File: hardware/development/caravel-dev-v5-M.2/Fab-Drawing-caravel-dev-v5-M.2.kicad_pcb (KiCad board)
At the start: 2 copper layers, 76.2 x 73.8 mm, 70 parts, among them J1 USB_B_Micro, J10 Conn_01x28_Pin, J11 Conn_01x28_Pin, J12 Conn_01x04_Pin, J2 Conn_01x02_Pin, J3 Conn_01x02_Pin, J4 Conn_01x03_Pin, J5 Conn_01x02_Pin, J6 Conn_01x02_Pin, J7 Conn_01x06_Pin, J8 Conn_01x02_Pin, J9 Conn_01x02_Pin, SW1 SW_Push - SKQGADE010, T1 Logo, T2 Logo, U1 FT232H, U2 SN74LVC1G125DCKR, U3 SN74LVC1G125DCKR, U5 TAR5SxxU, U6 TAR5SxxU, U7 W25Q32FVSS, U8 M.2-CONNECTOR-E, X1 DSC6001_10MHZ, Y1 12MHz

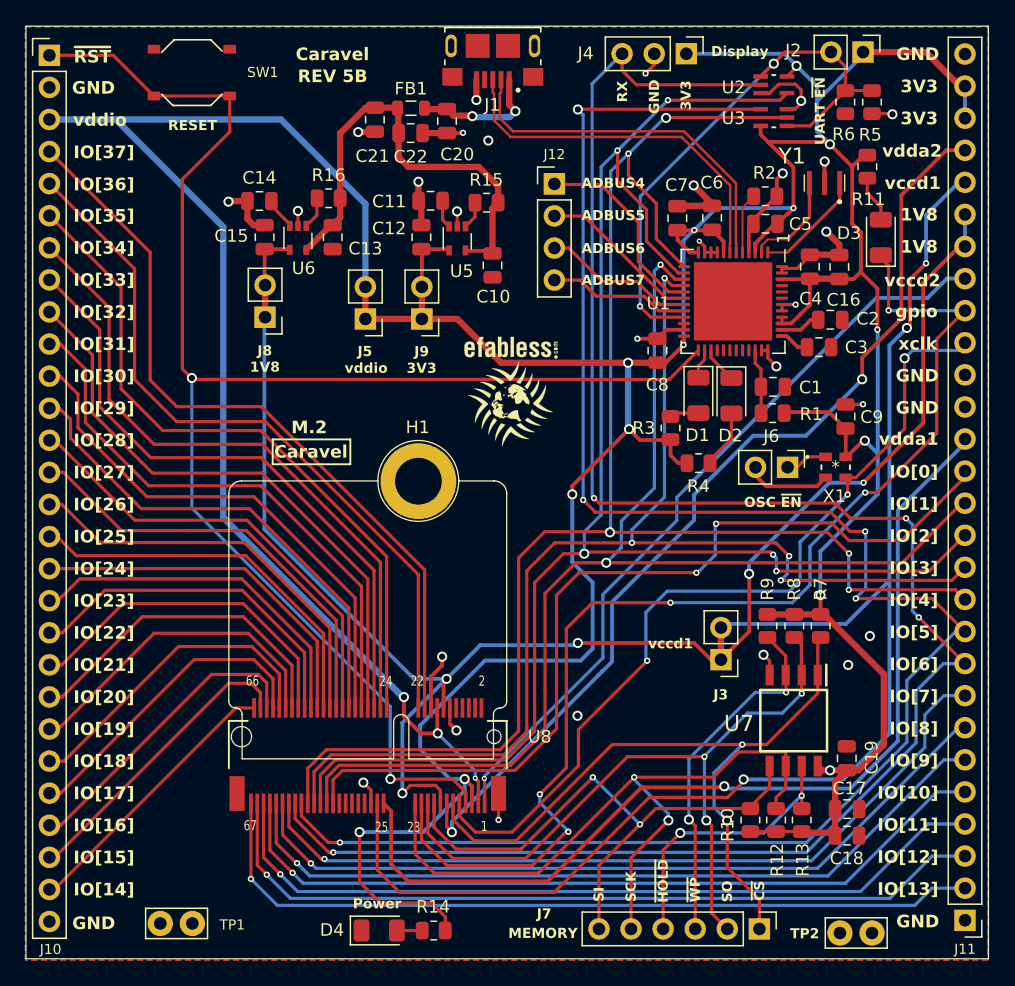
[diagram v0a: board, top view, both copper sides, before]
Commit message: ~ update caravel REV 5B PCB
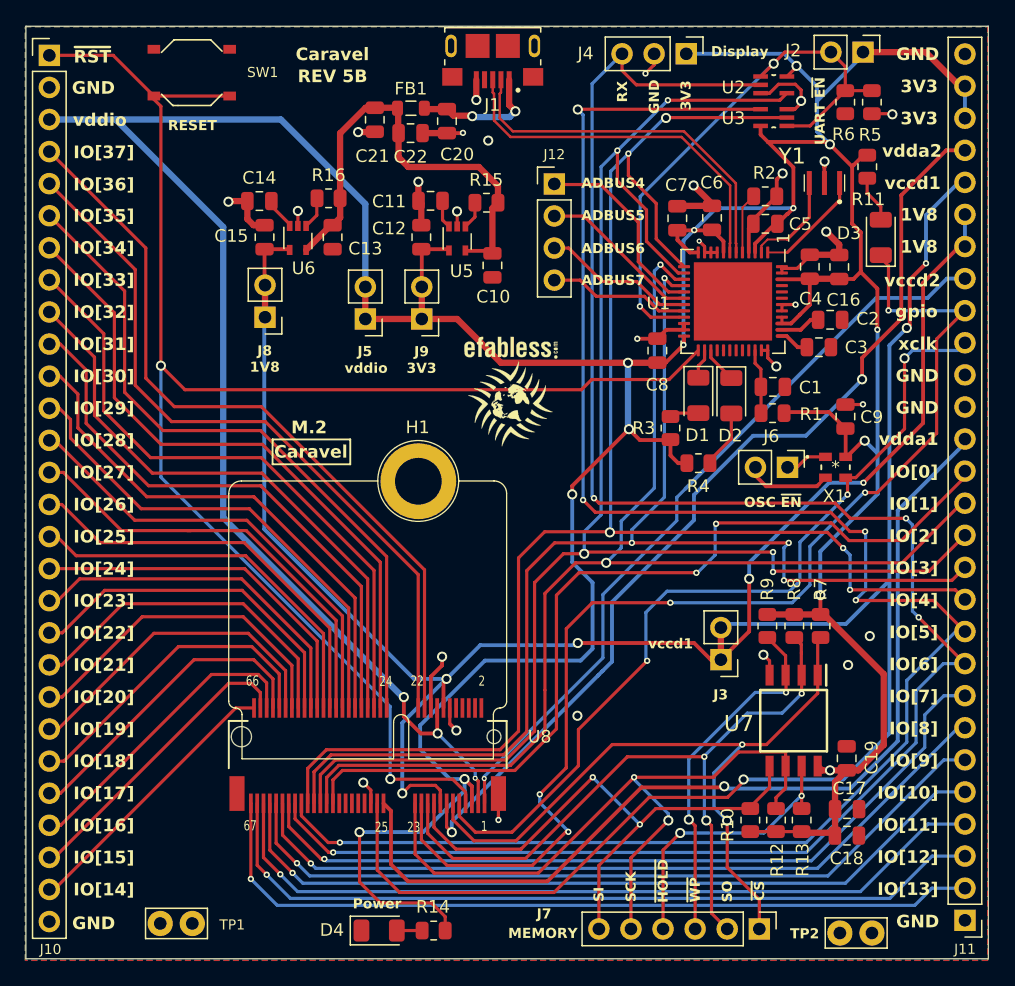
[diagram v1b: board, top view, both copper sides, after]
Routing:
- net /ACBUS1: track 126.3 -> 129.3 mm
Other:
- board text removed: "SW1"

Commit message: ~ update caravel REV 5B PCB
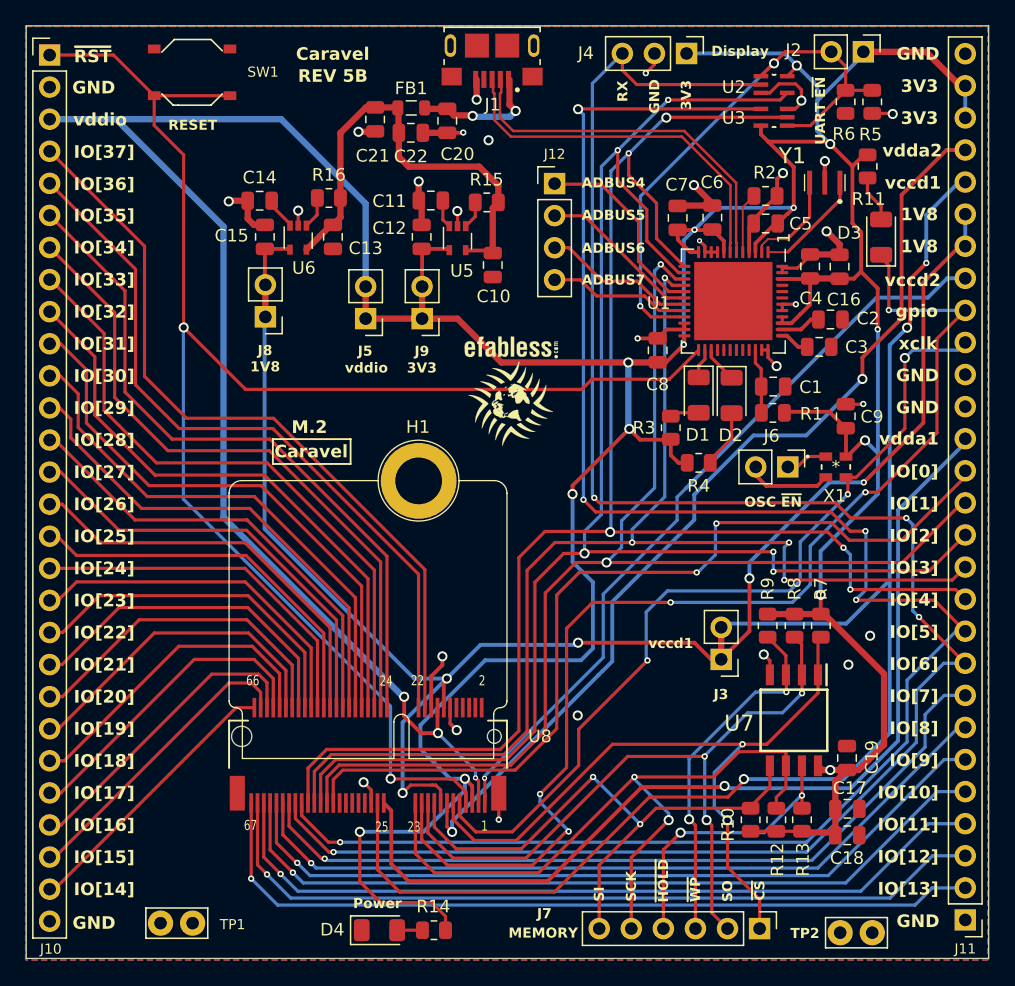
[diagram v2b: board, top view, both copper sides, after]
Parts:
- moved J1 0.06 mm to (131.9, 119.2)
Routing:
- net /ACBUS1: track 129.3 -> 128.8 mm
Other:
- board text added: "SW1"

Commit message: ~ enhance caravel REV 5B power tracks
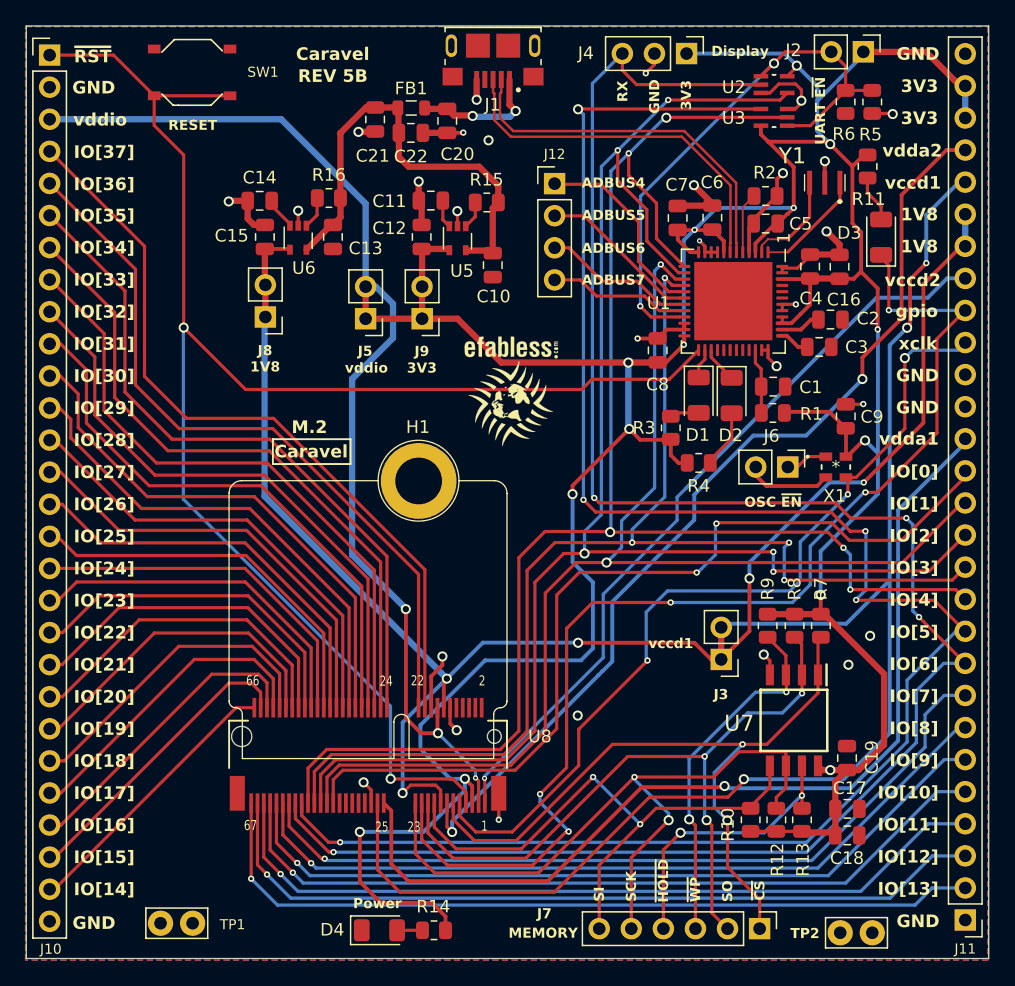
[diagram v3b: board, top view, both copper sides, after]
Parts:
- moved J1 0.08 mm to (132.0, 119.2)
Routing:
- net +3V3: track 403.3 -> 385.0 mm
- net +1V8: track 245.2 -> 243.7 mm
